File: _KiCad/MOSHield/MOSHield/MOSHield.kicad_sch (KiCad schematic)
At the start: 18 parts, among them J1 Power, J2 Digital/PWM, J3 Analog, J4 Digital/PWM, J5 Jumper, J7 Conn_01x08, U1 LTC1050

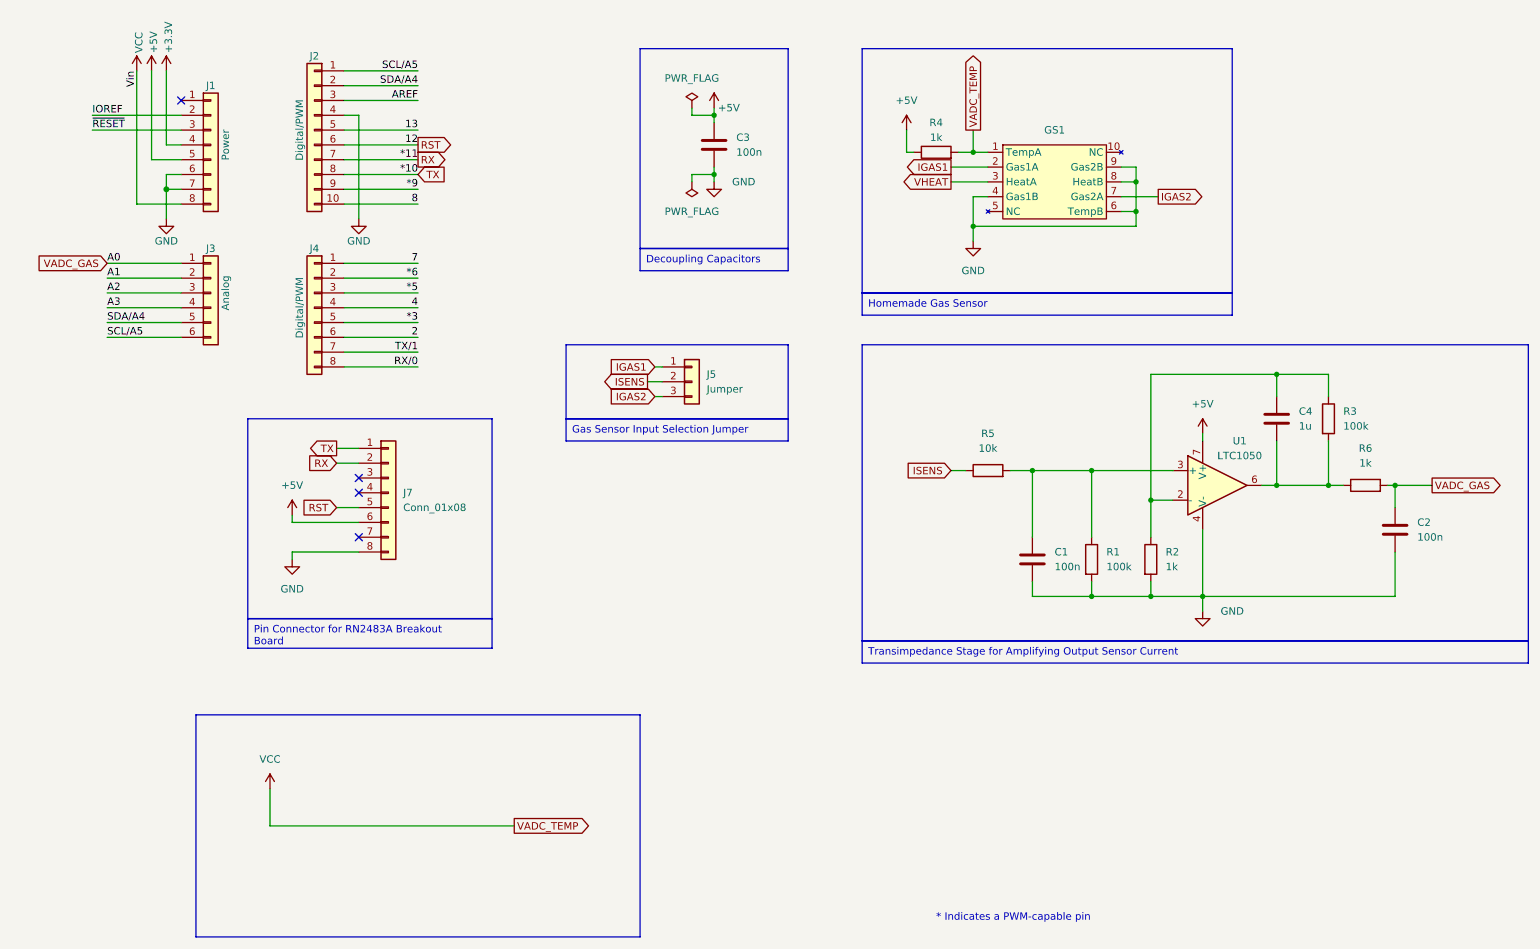
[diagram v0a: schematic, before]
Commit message: Added datasheet
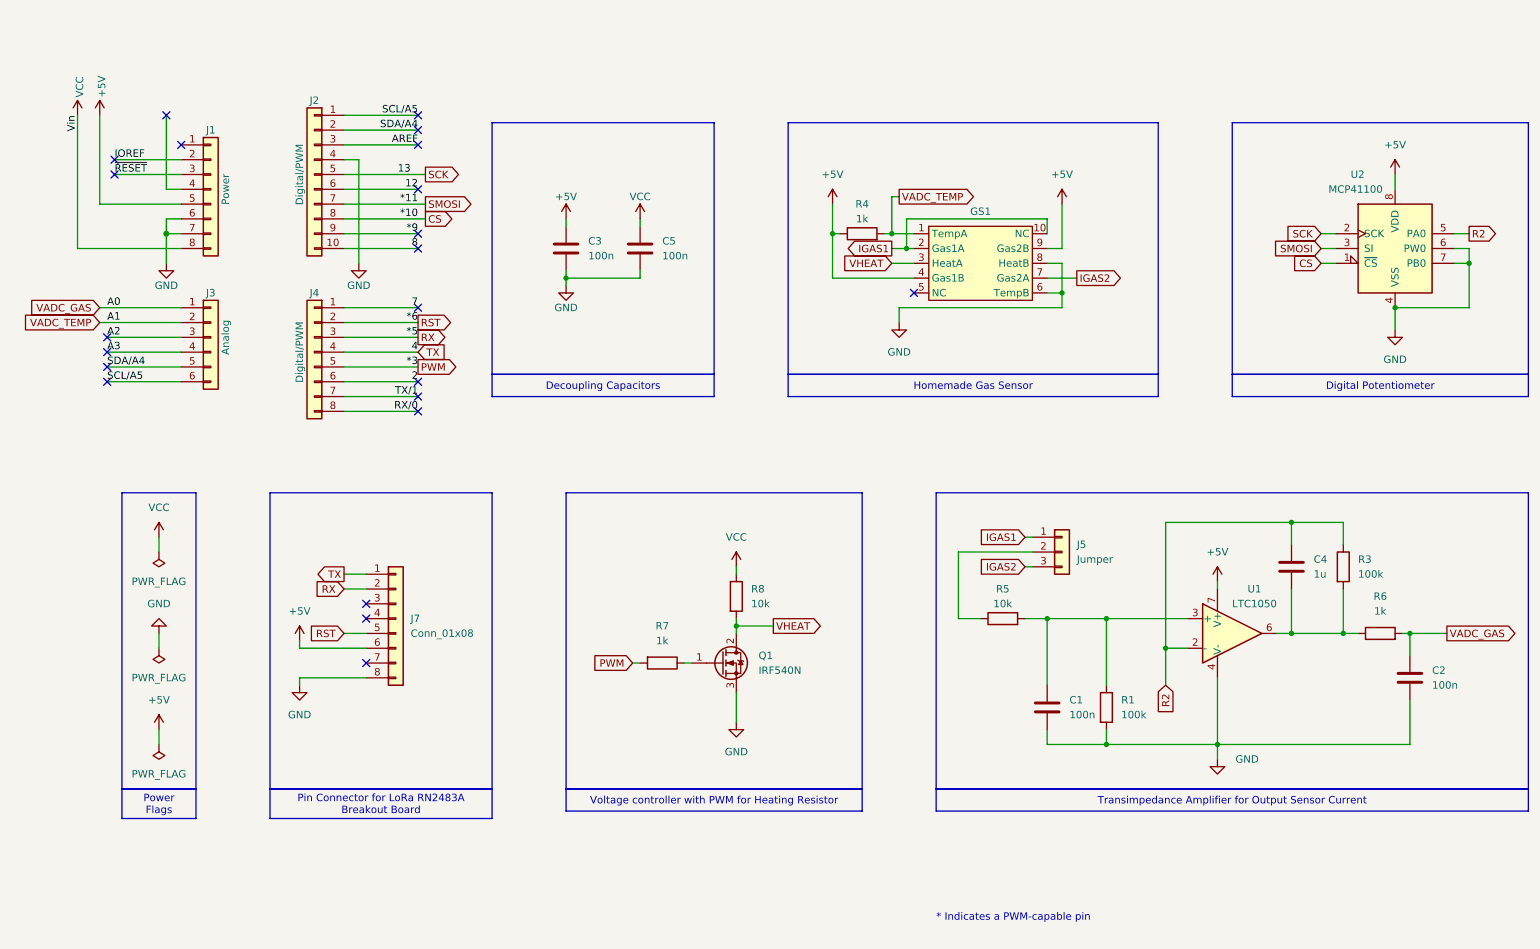
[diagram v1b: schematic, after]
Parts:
- removed R2: 1k, symbol Device:R
- added C5: 100n, Capacitor_THT:C_Disc_D4.7mm_W2.5mm_P5.00mm, symbol Device:C
- added Q1: IRF540N, Package_TO_SOT_THT:TO-220-3_Vertical, symbol Transistor_FET:IRF540N
- added R7: 1k, Resistor_THT:R_Axial_DIN0207_L6.3mm_D2.5mm_P10.16mm_Horizontal, symbol Device:R
- added R8: 10k, Resistor_THT:R_Axial_DIN0207_L6.3mm_D2.5mm_P10.16mm_Horizontal, symbol Device:R
- added U2: MCP41100, Package_DIP:DIP-8_W7.62mm, symbol Potentiometer_Digital:MCP41100
- C1, C2, C3: footprint (none) -> Capacitor_THT:C_Disc_D4.7mm_W2.5mm_P5.00mm
- C4: footprint (none) -> Capacitor_THT:C_Rect_L7.0mm_W4.5mm_P5.00mm
- J5: footprint (none) -> Connector_PinHeader_2.54mm:PinHeader_1x03_P2.54mm_Vertical
- R1, R3, R4, R5, R6: footprint (none) -> Resistor_THT:R_Axial_DIN0207_L6.3mm_D2.5mm_P10.16mm_Horizontal
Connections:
- net *5 is gone; now on net RX: J4.3 (Pin_3)
- net *6 is gone; now on net RST: J4.2 (Pin_2)
- net 4 is gone; now on net TX: J4.4 (Pin_4)
- net +5V: now also GS1.4 (Gas1B), GS1.9 (Gas2B), U2.8 (VDD)
- net GND: now also C5.2, Q1.3 (S), U2.4 (VSS), U2.6 (PW0), U2.7 (PB0); no longer GS1.4 (Gas1B), GS1.9 (Gas2B)
- net IGAS1: now also GS1.10 (NC)
- net RST: no longer J2.6 (Pin_6)
- net RX: no longer J2.7 (Pin_7)
- net TX: no longer J2.8 (Pin_8)
- net VCC: now also C5.1, R8.1; no longer GS1.1 (TempA), R4.2
- net VHEAT: now also Q1.2 (D), R8.2
- net R2: now reaches C4.1, R3.1, U1.2 (-)
- net R2: now also U2.5 (PA0)
- net *3 renamed PWM
- net PWM: now also R7.2
- net +3V3: no longer names the net of J1.4 (Pin_4)
- net 13 renamed SCK
- net SCK: now also U2.2 (SCK)
- net A1 renamed VADC_TEMP
- net VADC_TEMP: now also GS1.1 (TempA), R4.2
- net ISENS: no longer names the net of J5.2 (Pin_2), R5.1
- new net: Q1.1 (G), R7.1
- new net 12: J2.6 (Pin_6)
- new net CS: J2.8 (Pin_8), U2.1 (~{CS})
- new net SMOSI: J2.7 (Pin_7), U2.3 (SI)
- no-connect marks 4 -> 22
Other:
- moved on the sheet: C1, C2, C3, C4, J1, J2, J3, J4, J5, J7, R1, R3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
